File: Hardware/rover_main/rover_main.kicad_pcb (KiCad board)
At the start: 2 copper layers, 80 x 70 mm, 19 parts, among them J1 BATT, J2 BME280, J3 CSS811, J4 DRIVERS, J7 FTDI, J8 PROG, U1 LD1117A33, U2 MCP732831CHARGER, U3 ESP32-CAM

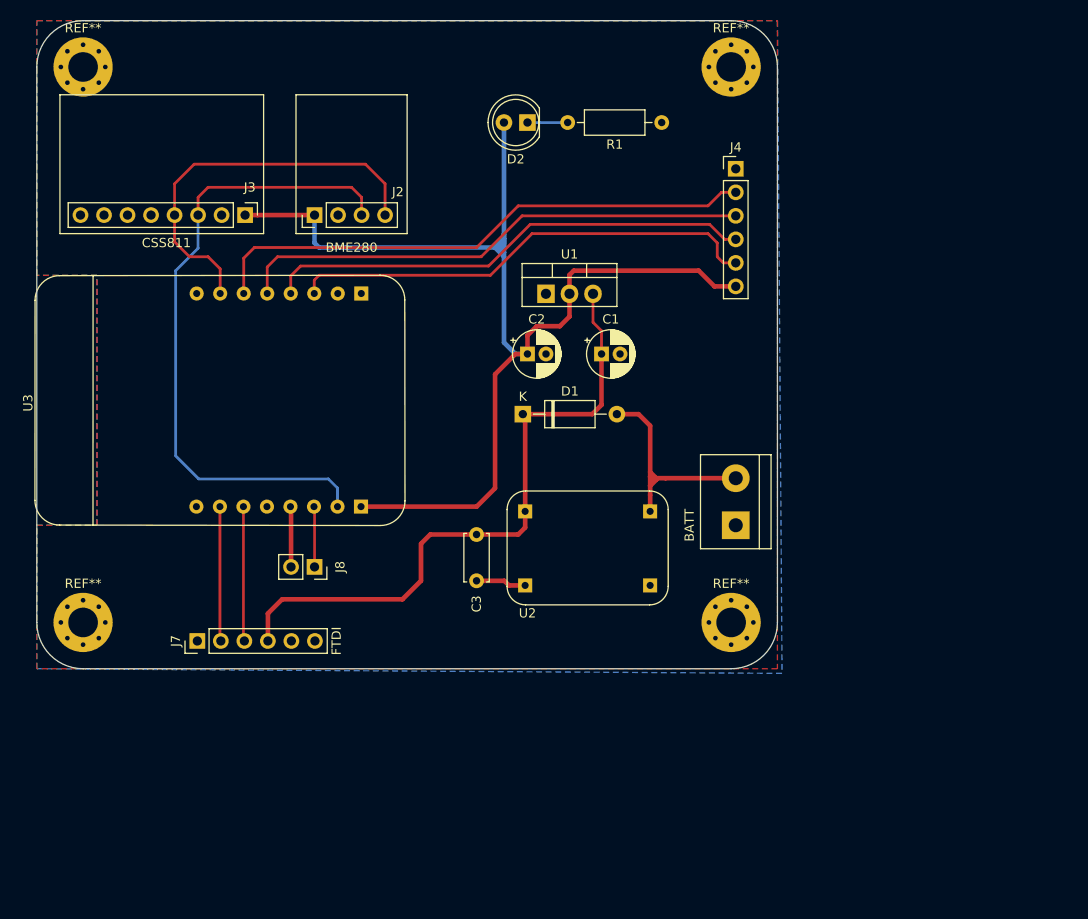
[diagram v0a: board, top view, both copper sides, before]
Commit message: Asig. places componets
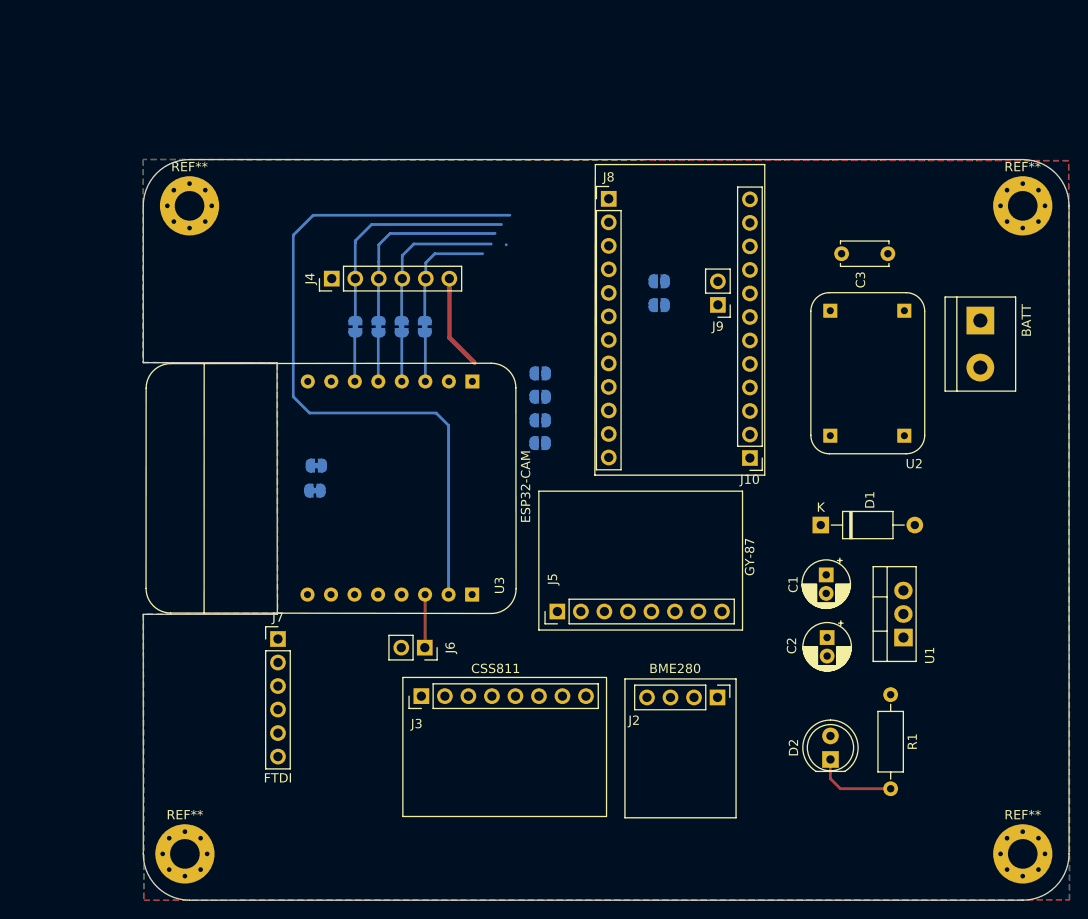
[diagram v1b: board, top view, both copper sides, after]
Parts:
- added J10: Analog, Connector_PinHeader_2.54mm:PinHeader_1x12_P2.54mm_Vertical, F.Cu at (167.0, 97.2)
- added J5: GY-87, Connector_PinHeader_2.54mm:PinHeader_1x08_P2.54mm_Vertical, F.Cu at (146.2, 113.8)
- added J6: PROG, Connector_PinSocket_2.54mm:PinSocket_1x02_P2.54mm_Vertical, F.Cu at (131.9, 117.7)
- added J9: i2c, Connector_PinHeader_2.54mm:PinHeader_1x02_P2.54mm_Vertical, F.Cu at (163.6, 80.7)
- added JP1: Engine 2B, Jumper:SolderJumper-2_P1.3mm_Bridged_RoundedPad1.0x1.5mm, B.Cu at (124.4, 83.0)
- added JP10: Engine 2B, Jumper:SolderJumper-2_P1.3mm_Open_RoundedPad1.0x1.5mm, B.Cu at (144.4, 88.1)
- added JP11: SDE ESP, Jumper:SolderJumper-2_P1.3mm_Bridged_RoundedPad1.0x1.5mm, B.Cu at (120.0, 100.8)
- added JP12: SCL ESP, Jumper:SolderJumper-2_P1.3mm_Bridged_RoundedPad1.0x1.5mm, B.Cu at (120.2, 98.1)
- added JP2: Engine 1A, Jumper:SolderJumper-2_P1.3mm_Bridged_RoundedPad1.0x1.5mm, B.Cu at (131.9, 83.0)
- added JP3: Engine 2A, Jumper:SolderJumper-2_P1.3mm_Bridged_RoundedPad1.0x1.5mm, B.Cu at (126.9, 83.0)
- added JP4: Engine 1B, Jumper:SolderJumper-2_P1.3mm_Bridged_RoundedPad1.0x1.5mm, B.Cu at (129.4, 83.0)
- added JP5: SDA, Jumper:SolderJumper-2_P1.3mm_Open_RoundedPad1.0x1.5mm, B.Cu at (157.2, 80.7)
- added JP6: SCL, Jumper:SolderJumper-2_P1.3mm_Open_RoundedPad1.0x1.5mm, B.Cu at (157.2, 78.2)
- added JP7: Engine 1A, Jumper:SolderJumper-2_P1.3mm_Open_RoundedPad1.0x1.5mm, B.Cu at (144.4, 93.2)
- added JP8: Engine 1B, Jumper:SolderJumper-2_P1.3mm_Open_RoundedPad1.0x1.5mm, B.Cu at (144.4, 95.6)
- added JP9: Engine 2A, Jumper:SolderJumper-2_P1.3mm_Open_RoundedPad1.0x1.5mm, B.Cu at (144.4, 90.6)
- J8: value PROG -> Digital; footprint Connector_PinSocket_2.54mm:PinSocket_1x02_P2.54mm_Vertical -> Connector_PinHeader_2.54mm:PinHeader_1x12_P2.54mm_Vertical
- moved D2 76.2 mm to (175.7, 129.8), turned to 90 degrees
- moved J2 67.9 mm to (163.5, 123.1), turned to 270 degrees
- moved R1 66.6 mm to (182.2, 122.8), turned to 270 degrees
- moved J3 55.3 mm to (131.5, 123.0), turned to 90 degrees
- moved C3 53.8 mm to (181.9, 75.2), turned to 180 degrees
- moved U1 53.6 mm to (183.6, 116.6), turned to 90 degrees
- moved J8 50.9 mm to (151.8, 69.2), turned to 0 degrees
- moved J4 45.2 mm to (121.9, 77.9), turned to 90 degrees
- moved C2 44.6 mm to (175.4, 116.6), turned to 270 degrees
- moved REF** 40.2 mm to (196.5, 140.0)
- moved U2 35.6 mm to (179.7, 88.1), turned to 0 degrees
- moved REF** 34.9 mm to (196.5, 70.0)
- moved J1 34.5 mm to (191.9, 82.4), turned to 270 degrees
- moved D1 34.3 mm to (174.7, 104.5)
- moved C1 34.0 mm to (175.3, 109.9), turned to 270 degrees
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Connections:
- J8 pad 1: /GPIO0 -> /RX
- J8 pad 2: GND -> /TX
- U3 pad 11: /GPIO12 -> /GPIO12E
- U3 pad 12: /GPIO13 -> /GPIO13E
- U3 pad 13: /GPIO15 -> /GPIO15E
- U3 pad 14: /GPIO14 -> /GPIO14E
- U3 pad 15: /SDA -> /SDAE
- U3 pad 7: /SCL -> /SCLE
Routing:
- net +3V3: track 126.8 -> 10.6 mm
- net /SCLE: track 0.00 -> 78.1 mm
- net VCC: track 70.6 -> 0.00 mm
- net /SCL: track 70.3 -> 0.00 mm
- net /SDA: track 42.9 -> 0.00 mm
- net /GPIO12: track 51.2 -> 12.8 mm
- net /GPIO13: track 52.9 -> 17.2 mm
- net /GPIO14: track 59.9 -> 25.1 mm
- net /GPIO15: track 55.8 -> 21.3 mm
- net /BATT: track 24.7 -> 0.00 mm
- net /RX: track 14.6 -> 0.00 mm
- net /TX: track 14.6 -> 0.00 mm
- net GND: track 12.0 -> 0.00 mm
- net /GPIO14E: track 0.00 -> 5.29 mm
- net /GPIO12E: track 0.00 -> 5.29 mm
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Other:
- board size 80 x 70 mm -> 100 x 80 mm

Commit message: RE-ROUTEO
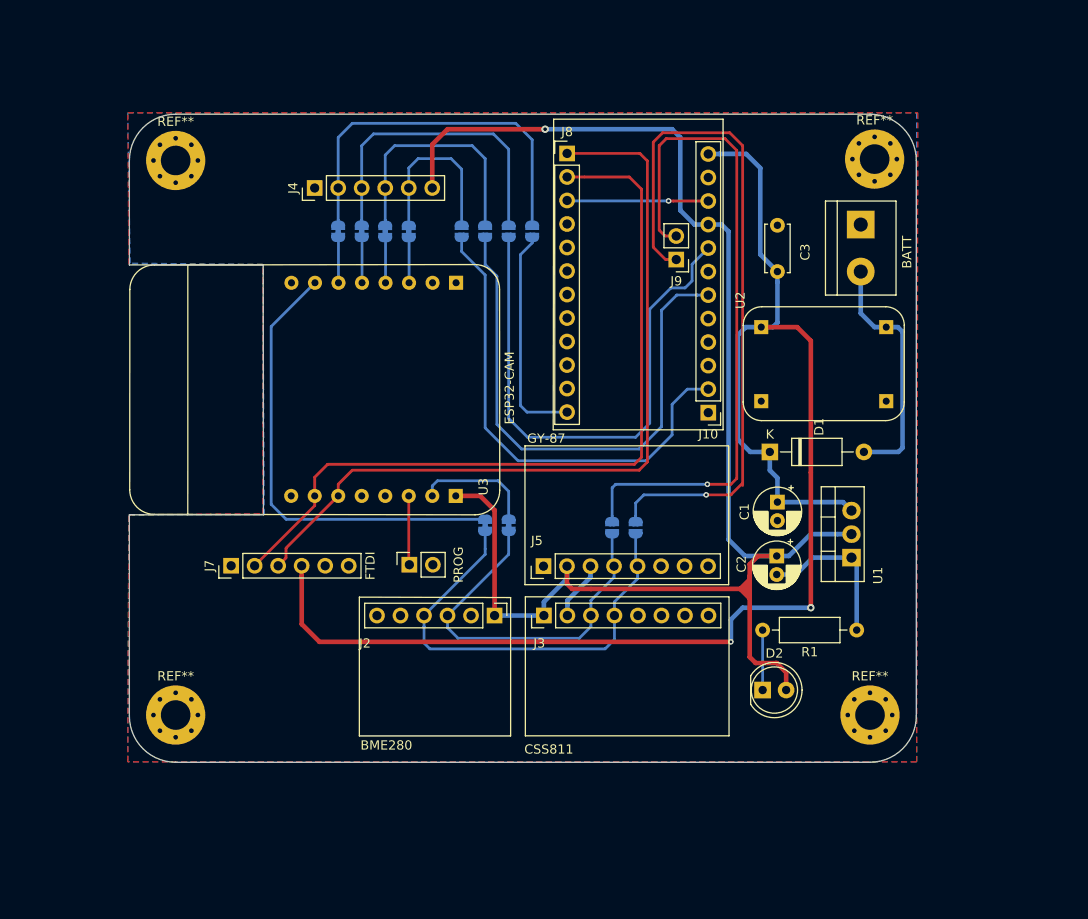
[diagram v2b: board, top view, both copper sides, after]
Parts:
- removed the REF** at (106.0, 140.0)
- removed the REF** at (106.5, 70.0)
- removed the REF** at (196.5, 70.0)
- removed the REF** at (196.5, 140.0)
- added REF**: MountingHole_3.2mm_M3_Pad_Via, MountingHole:MountingHole_3.2mm_M3_Pad_Via, F.Cu at (105.0, 125.0)
- added REF**: MountingHole_3.2mm_M3_Pad_Via, MountingHole:MountingHole_3.2mm_M3_Pad_Via, F.Cu at (105.0, 65.1)
- added REF**: MountingHole_3.2mm_M3_Pad_Via, MountingHole:MountingHole_3.2mm_M3_Pad_Via, F.Cu at (180.5, 65.0)
- added REF**: MountingHole_3.2mm_M3_Pad_Via, MountingHole:MountingHole_3.2mm_M3_Pad_Via, F.Cu at (180.0, 125.0)
- J2: footprint Connector_PinHeader_2.54mm:PinHeader_1x04_P2.54mm_Vertical -> Connector_PinHeader_2.54mm:PinHeader_1x06_P2.54mm_Vertical
- moved JP6 27.1 mm to (152.1, 104.8), turned to 270 degrees
- moved J2 25.7 mm to (139.4, 114.3)
- moved JP8 24.4 mm to (135.9, 72.8), turned to 90 degrees
- moved JP5 24.2 mm to (154.7, 104.8), turned to 270 degrees
- moved JP12 21.7 mm to (141.0, 104.5), turned to 270 degrees
- moved JP7 21.3 mm to (138.4, 72.8), turned to 90 degrees
- moved JP11 18.8 mm to (138.4, 104.5), turned to 270 degrees
- moved JP9 18.2 mm to (141.0, 72.8), turned to 90 degrees
- moved J1 16.6 mm to (179.0, 72.0)
- moved J3 15.8 mm to (144.8, 114.2)
- moved JP10 15.4 mm to (143.5, 72.8), turned to 90 degrees
- moved C3 12.1 mm to (170.0, 77.1), turned to 90 degrees
- moved U3 10.8 mm to (124.7, 89.8)
- moved D2 10.5 mm to (168.4, 122.3), turned to 0 degrees
- moved JP1 10.5 mm to (122.6, 72.8)
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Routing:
- net +3V3: track 10.6 -> 168.8 mm, vias 0 -> 1
- net VCC: track 0.00 -> 157.8 mm, vias 0 -> 2
- net /RX: track 0.00 -> 87.4 mm
- net /TX: track 0.00 -> 86.0 mm
- net /SDAB: track 0.00 -> 76.2 mm, vias 0 -> 1
- net /SCLB: track 0.00 -> 73.4 mm, vias 0 -> 1
- net /SCLE: track 78.1 -> 13.1 mm
- net /A1: track 0.00 -> 58.9 mm
- net /A3: track 0.00 -> 58.7 mm
- net /11: track 0.00 -> 52.3 mm
- net /SDAE: track 0.00 -> 49.7 mm
- net /SDA: track 0.00 -> 48.6 mm
- net /SCL: track 0.00 -> 40.8 mm
- net /BATT: track 0.00 -> 26.7 mm
- net /9: track 0.00 -> 24.0 mm
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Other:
- board size 100 x 80 mm -> 85 x 70 mm
